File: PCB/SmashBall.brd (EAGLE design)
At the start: 101.6 x 101.6 mm, 12 parts

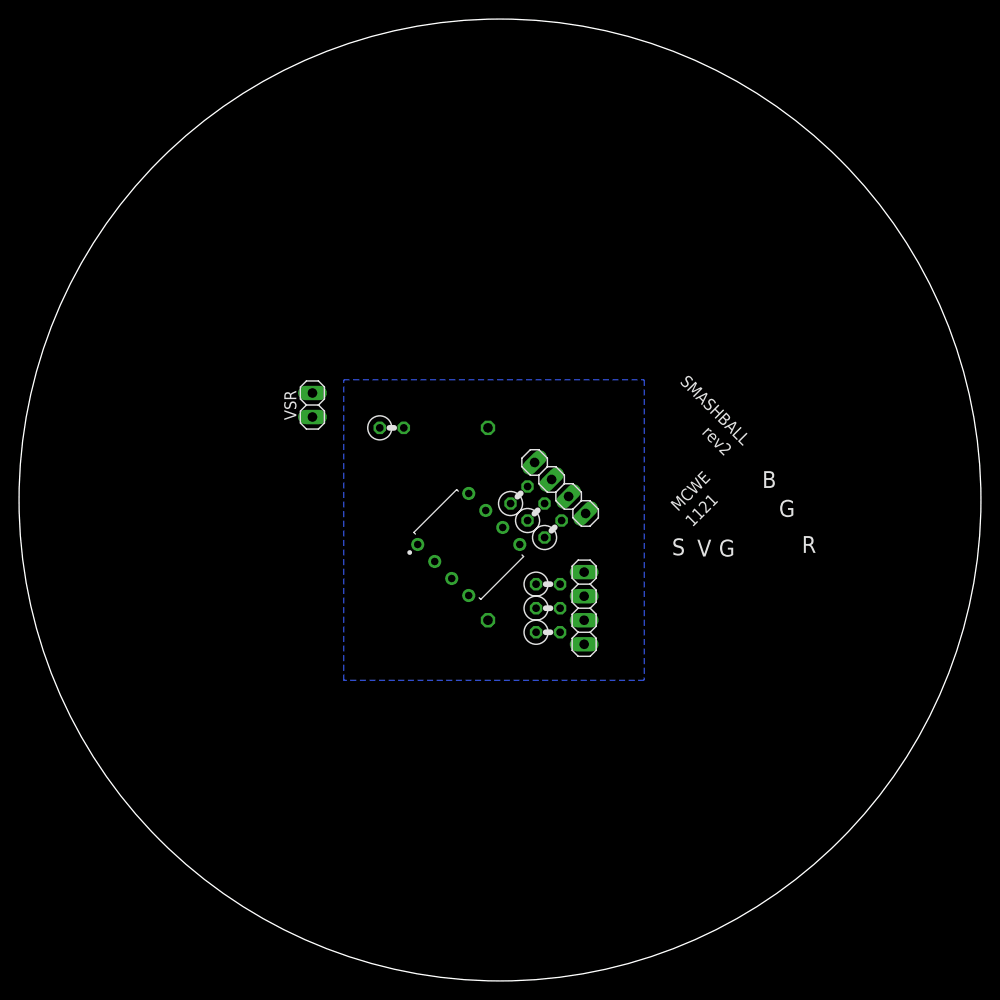
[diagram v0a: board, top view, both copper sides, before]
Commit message: Finished layout of the board.
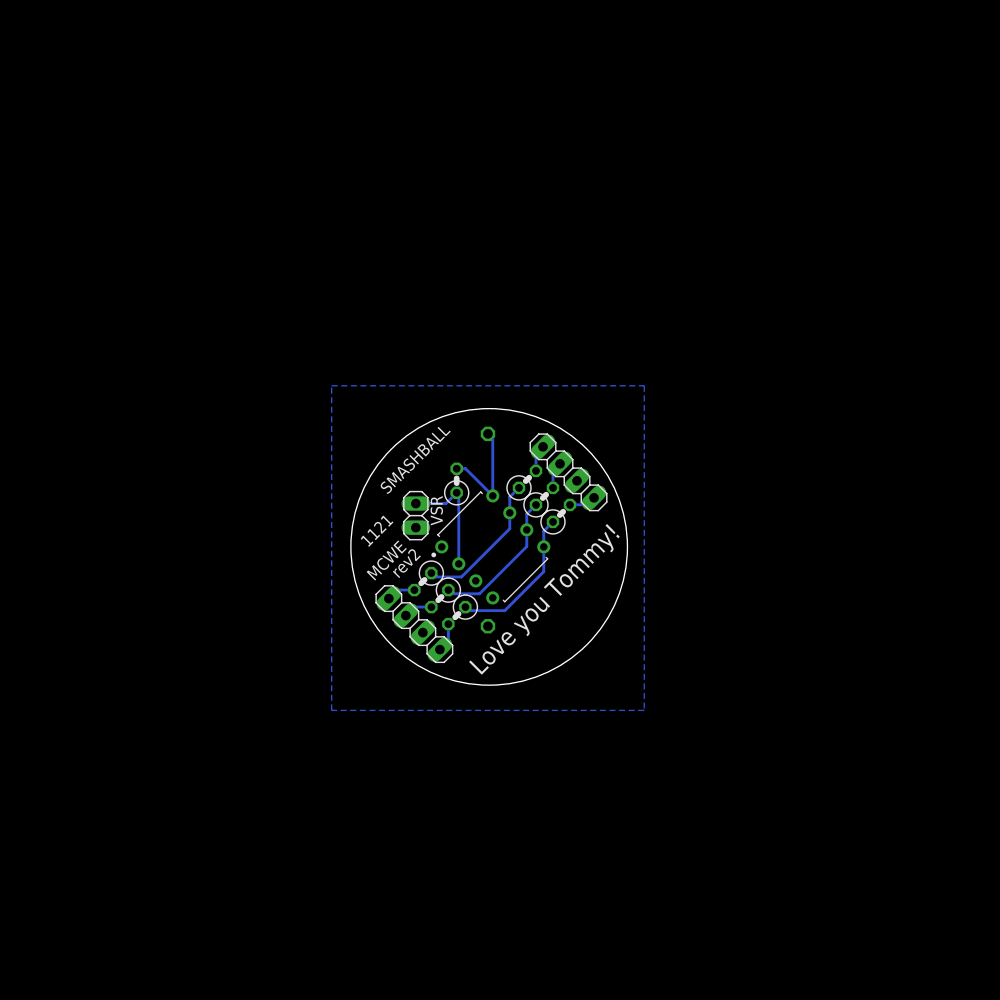
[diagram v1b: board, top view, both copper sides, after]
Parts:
- moved RGB_LED2 18.0 mm to (-7.77, -8.03), turned to 135 degrees
- moved VSR 16.0 mm to (-7.62, 3.43), turned to 270 degrees
- moved R6 14.3 mm to (-6.88, -3.54), turned to 225 degrees
- moved R5 11.5 mm to (-5.08, -5.33), turned to 225 degrees
- moved R4 10.2 mm to (-3.28, -7.13), turned to 225 degrees
- moved R7 8.85 mm to (-3.30, 7.11), turned to 90 degrees
- moved U$1 2.55 mm to (0.51, 0.13)
- moved R2 1.88 mm to (5.97, 5.46)
- moved R1 1.88 mm to (7.77, 3.66)
- moved R3 1.88 mm to (4.17, 7.26)
- moved RGB_LED1 1.88 mm to (8.51, 8.00)
- moved U$2 0.64 mm to (0.00, -8.26)
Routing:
- net RED: track 0.00 -> 15.8 mm
- net GREEN: track 0.00 -> 15.3 mm
- net BLUE: track 0.00 -> 15.3 mm
- net SWTCH: track 0.00 -> 12.4 mm
- net VIN: track 0.00 -> 11.8 mm
- net RED2: track 0.00 -> 3.07 mm
- net GREEN2: track 0.00 -> 3.07 mm
- net BLUE2: track 0.00 -> 3.07 mm
- net BLUE1: track 0.00 -> 2.85 mm
- net GREEN1: track 0.00 -> 2.85 mm
- net RED1: track 0.00 -> 2.39 mm
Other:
- board size 101.6 x 101.6 mm -> 29.2 x 29.2 mm
- board text added: "Love you Tommy!"
- board text removed: "B"
- board text removed: "G"
- board text removed: "R"
- board text removed: "S"
- board text removed: "V"
